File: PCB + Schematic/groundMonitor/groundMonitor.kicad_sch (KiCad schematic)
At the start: 26 parts, among them J1 FTDI, J2 Header, J3 5-12 V, J4 USB-C, J5 Power, SW1 Boot, SW2 EN, U1 ESP32-C3-MINI-1-N4, U2 Ra-01, U3 AMS1117-3.3

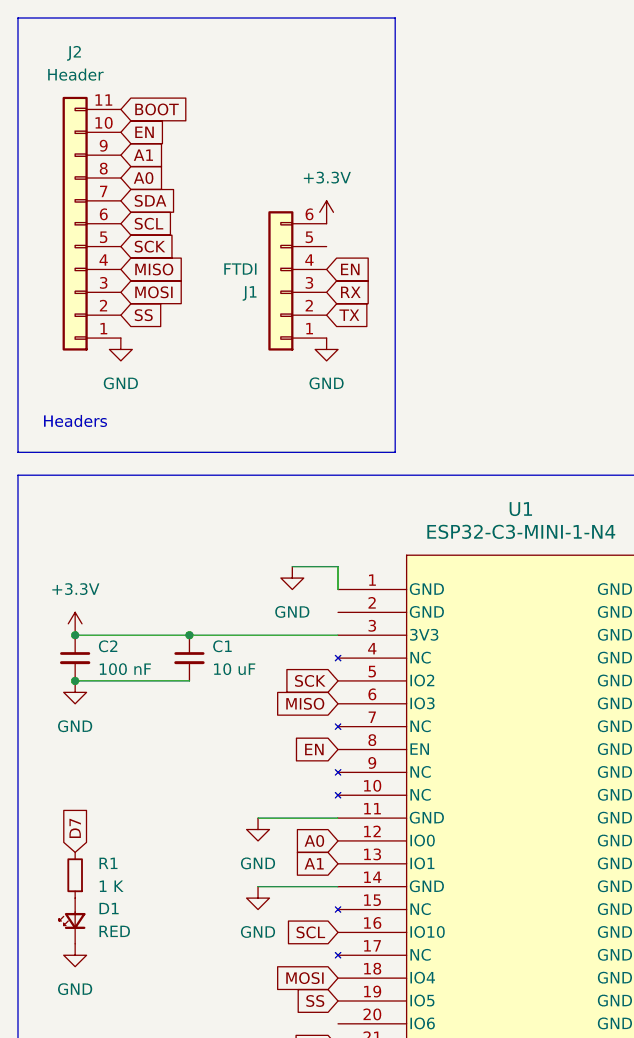
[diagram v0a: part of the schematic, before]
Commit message: PCB!
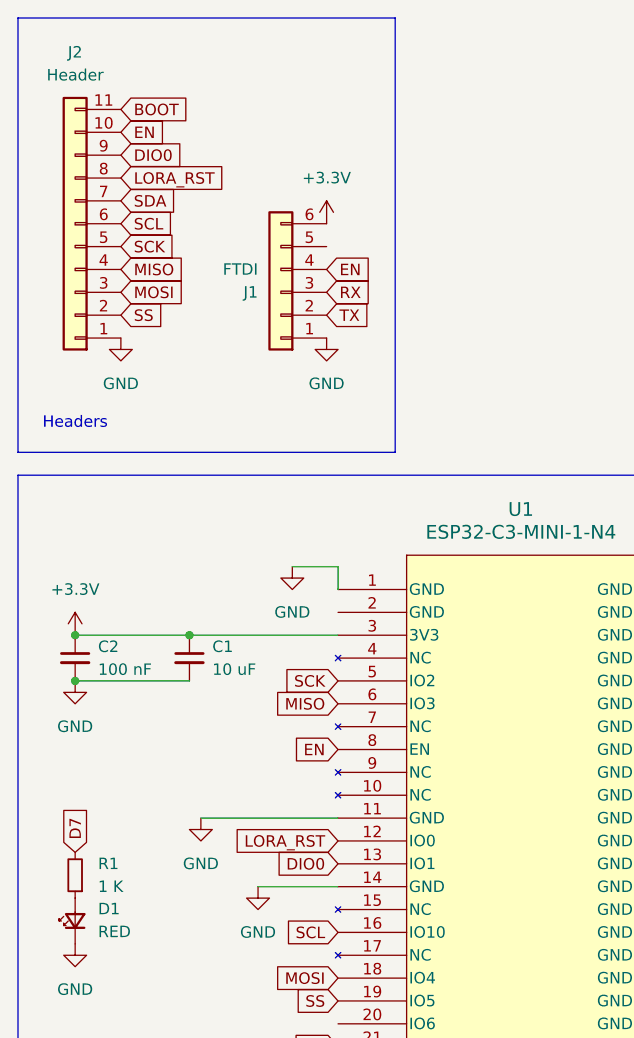
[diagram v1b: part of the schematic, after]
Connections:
- net A0 is gone; now on net LORA_RST: J2.8 (Pin_8), U1.12 (IO0)
- net A1 is gone; now on net DIO0: J2.9 (Pin_9), U1.13 (IO1)
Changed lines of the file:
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@@
 	(wire
 		(pts
-			(xy 41.91 138.43) (xy 50.8 138.43)
+			(xy 35.56 138.43) (xy 50.8 138.43)
 		)
 		(stroke
@@
 		)
 	)
+	(global_label "LORA_RST"
+		(shape input)
+		(at 26.67 67.31 0)
+		(fields_autoplaced yes)
+		(effects
+			(font
+				(size 1.27 1.27)
+			)
+			(justify left)
+		)
+		(property "Intersheetrefs" "${INTERSHEET_REFS}"
+			(at 38.7871 67.31 0)
+			(effects
+				(font
+					(size 1.27 1.27)
+				)
+				(justify left)
+				(hide yes)
+			)
+		)
+	)
 	(global_label "BOOT"
 		(shape input)
@@
 		)
 	)
+	(global_label "DIO0"
+		(shape input)
+		(at 26.67 64.77 0)
+		(fields_autoplaced yes)
+		(effects
+			(font
+				(size 1.27 1.27)
+			)
+			(justify left)
+		)
+		(property "Intersheetrefs" "${INTERSHEET_REFS}"
+			(at 34.07 64.77 0)
+			(effects
+				(font
+					(size 1.27 1.27)
+				)
+				(justify left)
+				(hide yes)
+			)
+		)
+	)
 	(global_label "D7"
 		(shape input)
@@
 		)
 	)
+	(global_label "LORA_RST"
+		(shape input)
+		(at 50.8 140.97 180)
+		(fields_autoplaced yes)
+		(effects
+			(font
+				(size 1.27 1.27)
+			)
+			(justify right)
+		)
+		(property "Intersheetrefs" "${INTERSHEET_REFS}"
+			(at 38.6829 140.97 0)
+			(effects
+				(font
+					(size 1.27 1.27)
+				)
+				(justify right)
+				(hide yes)
+			)
+		)
+	)
 	(global_label "RX"
 		(shape input)
@@
 		)
 	)
-	(global_label "A1"
-		(shape input)
-		(at 26.67 64.77 0)
-		(fields_autoplaced yes)
-		(effects
-			(font
-				(size 1.27 1.27)
-			)
-			(justify left)
-		)
-		(property "Intersheetrefs" "${INTERSHEET_REFS}"
-			(at 31.9533 64.77 0)
-			(effects
-				(font
-					(size 1.27 1.27)
-				)
-				(justify left)
-				(hide yes)
-			)
-		)
-	)
-	(global_label "A1"
+	(global_label "DIO0"
 		(shape input)
 		(at 50.8 143.51 180)
@@
 		)
 		(property "Intersheetrefs" "${INTERSHEET_REFS}"
-			(at 45.5167 143.51 0)
+			(at 43.4 143.51 0)
 			(effects
 				(font
@@
 		(property "Intersheetrefs" "${INTERSHEET_REFS}"
 			(at 45.3353 186.69 0)
-			(effects
-				(font
-					(size 1.27 1.27)
-				)
-				(justify right)
-				(hide yes)
-			)
-		)
-	)
-	(global_label "A0"
-		(shape input)
-		(at 26.67 67.31 0)
-		(fields_autoplaced yes)
-		(effects
-			(font
-				(size 1.27 1.27)
-			)
-			(justify left)
-		)
-		(property "Intersheetrefs" "${INTERSHEET_REFS}"
-			(at 31.9533 67.31 0)
-			(effects
-				(font
-					(size 1.27 1.27)
-				)
-				(justify left)
-				(hide yes)
-			)
-		)
-	)
-	(global_label "A0"
-		(shape input)
-		(at 50.8 140.97 180)
-		(fields_autoplaced yes)
-		(effects
-			(font
-				(size 1.27 1.27)
-			)
-			(justify right)
-		)
-		(property "Intersheetrefs" "${INTERSHEET_REFS}"
-			(at 45.5167 140.97 0)
 			(effects
 				(font
@@
 	(symbol
 		(lib_id "power:GND")
-		(at 41.91 138.43 0)
+		(at 35.56 138.43 0)
 		(unit 1)
 		(exclude_from_sim no)
@@
 		(fields_autoplaced yes)
 		(property "Reference" "#PWR014"
-			(at 41.91 144.78 0)
+			(at 35.56 144.78 0)
 			(effects
 				(font
@@
 		)
 		(property "Value" "GND"
-			(at 41.91 143.51 0)
+			(at 35.56 143.51 0)
 			(effects
 				(font
@@
 		)
 		(property "Footprint" ""
-			(at 41.91 138.43 0)
+			(at 35.56 138.43 0)
 			(effects
 				(font
@@
 		)
 		(property "Datasheet" ""
-			(at 41.91 138.43 0)
+			(at 35.56 138.43 0)
 			(effects
 				(font
@@
 		)
 		(property "Description" "Power symbol creates a global label with name \"GND\" , ground"
-			(at 41.91 138.43 0)
-			(effects
-				(font
+			(at 35.56 138.43 0)
+			(effects
+				(font
